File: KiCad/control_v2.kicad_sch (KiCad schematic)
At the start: 22 parts, among them J1 DE9_Pins, J2 DE9_Pins, J3 Conn_01x05, U1 FDC2214, U2 SN65HVD230, U3 PIC24HJ128GP502, Y1 Crystal

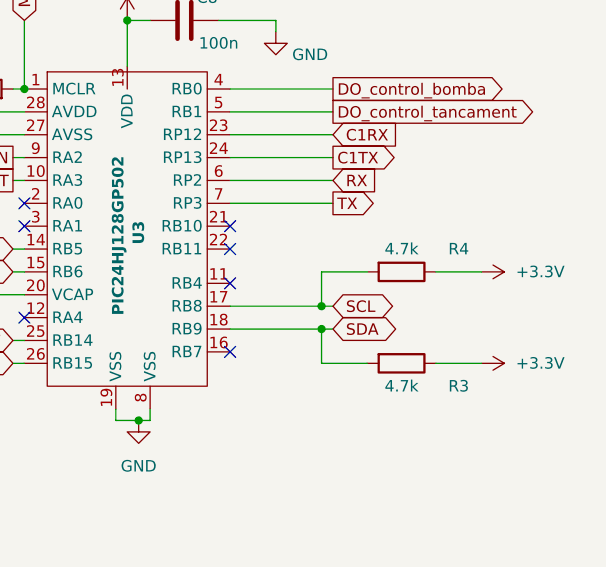
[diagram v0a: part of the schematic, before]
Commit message: commit por alfred
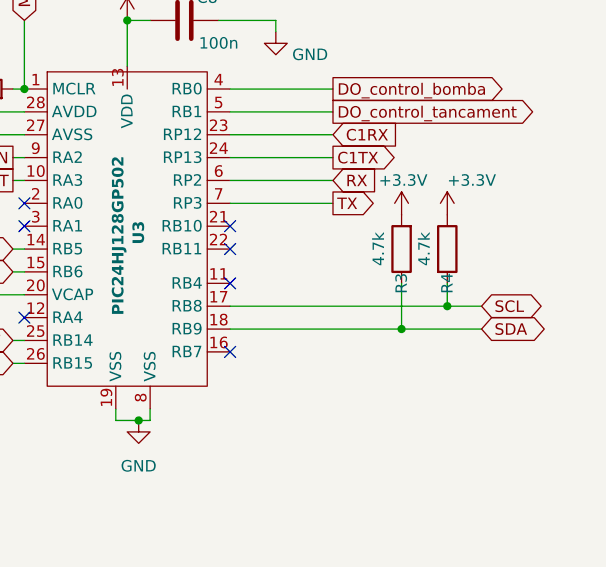
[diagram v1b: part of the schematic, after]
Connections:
- net +3.3V: now also R3.2; no longer R3.1
- net SDA: now also R3.1; no longer R3.2
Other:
- moved on the sheet: R3, R4
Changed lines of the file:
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@@
 	)
 	(junction
-		(at 231.14 68.58)
-		(diameter 0)
-		(color 0 0 0 0)
-	)
-	(junction
 		(at 100.33 60.96)
 		(diameter 0)
@@
 	)
 	(junction
+		(at 240.03 68.58)
+		(diameter 0)
+		(color 0 0 0 0)
+	)
+	(junction
 		(at 217.17 123.19)
 		(diameter 0)
@@
 	)
 	(junction
-		(at 231.14 66.04)
+		(at 245.11 66.04)
 		(diameter 0)
 		(color 0 0 0 0)
@@
 	(wire
 		(pts
-			(xy 236.22 72.39) (xy 231.14 72.39)
-		)
-		(stroke
-			(width 0)
-			(type default)
-		)
-	)
-	(wire
-		(pts
 			(xy 208.28 78.74) (xy 210.82 78.74)
 		)
@@
 	(wire
 		(pts
-			(xy 236.22 62.23) (xy 231.14 62.23)
-		)
-		(stroke
-			(width 0)
-			(type default)
-		)
-	)
-	(wire
-		(pts
-			(xy 243.84 72.39) (xy 248.92 72.39)
+			(xy 160.02 120.65) (xy 165.1 120.65)
 		)
 		(stroke
@@
 	(wire
 		(pts
-			(xy 160.02 120.65) (xy 165.1 120.65)
+			(xy 240.03 68.58) (xy 248.92 68.58)
 		)
 		(stroke
@@
 	(wire
 		(pts
-			(xy 220.98 66.04) (xy 231.14 66.04)
+			(xy 220.98 66.04) (xy 245.11 66.04)
 		)
 		(stroke
@@
 	(wire
 		(pts
+			(xy 245.11 63.5) (xy 245.11 66.04)
+		)
+		(stroke
+			(width 0)
+			(type default)
+		)
+	)
+	(wire
+		(pts
 			(xy 219.71 34.29) (xy 226.06 34.29)
 		)
@@
 	(wire
 		(pts
-			(xy 220.98 49.53) (xy 232.41 49.53)
+			(xy 245.11 66.04) (xy 248.92 66.04)
 		)
 		(stroke
@@
 	(wire
 		(pts
-			(xy 184.15 40.64) (xy 184.15 44.45)
+			(xy 220.98 49.53) (xy 232.41 49.53)
 		)
 		(stroke
@@
 	(wire
 		(pts
-			(xy 184.15 46.99) (xy 184.15 48.26)
+			(xy 184.15 40.64) (xy 184.15 44.45)
 		)
 		(stroke
@@
 	(wire
 		(pts
-			(xy 243.84 62.23) (xy 248.92 62.23)
+			(xy 184.15 46.99) (xy 184.15 48.26)
 		)
 		(stroke
@@
 	(wire
 		(pts
-			(xy 220.98 68.58) (xy 231.14 68.58)
+			(xy 220.98 68.58) (xy 240.03 68.58)
 		)
 		(stroke
@@
 	(wire
 		(pts
+			(xy 240.03 63.5) (xy 240.03 68.58)
+		)
+		(stroke
+			(width 0)
+			(type default)
+		)
+	)
+	(wire
+		(pts
 			(xy 160.02 128.27) (xy 165.1 128.27)
 		)
@@
 		)
 	)
-	(wire
-		(pts
-			(xy 231.14 66.04) (xy 232.41 66.04)
-		)
-		(stroke
-			(width 0)
-			(type default)
-		)
-	)
 	(bus
 		(pts
@@
 	(wire
 		(pts
-			(xy 231.14 68.58) (xy 231.14 72.39)
-		)
-		(stroke
-			(width 0)
-			(type default)
-		)
-	)
-	(wire
-		(pts
 			(xy 102.87 151.13) (xy 105.41 151.13)
 		)
@@
 	(wire
 		(pts
-			(xy 231.14 68.58) (xy 232.41 68.58)
-		)
-		(stroke
-			(width 0)
-			(type default)
-		)
-	)
-	(wire
-		(pts
 			(xy 100.33 60.96) (xy 106.68 60.96)
 		)
@@
 	(wire
 		(pts
-			(xy 231.14 62.23) (xy 231.14 66.04)
-		)
-		(stroke
-			(width 0)
-			(type default)
-		)
-	)
-	(wire
-		(pts
 			(xy 96.52 53.34) (xy 100.33 53.34)
 		)
@@
 	(global_label "SDA"
 		(shape bidirectional)
-		(at 232.41 68.58 0)
+		(at 248.92 68.58 0)
 		(fields_autoplaced yes)
 		(effects
@@
 		)
 		(property "Intersheetrefs" "${INTERSHEET_REFS}"
-			(at 240.0746 68.58 0)
+			(at 256.5846 68.58 0)
 			(effects
 				(font
@@
 	(global_label "SCL"
 		(shape bidirectional)
-		(at 232.41 66.04 0)
+		(at 248.92 66.04 0)
 		(fields_autoplaced yes)
 		(effects
@@
 		)
 		(property "Intersheetrefs" "${INTERSHEET_REFS}"
-			(at 240.0141 66.04 0)
+			(at 256.5241 66.04 0)
 			(effects
 				(font
@@
 	(symbol
 		(lib_id "power:+3.3V")
-		(at 248.92 62.23 270)
+		(at 245.11 55.88 0)
 		(unit 1)
 		(exclude_from_sim no)
@@
 		(on_board yes)
 		(dnp no)
-		(fields_autoplaced yes)
 		(property "Reference" "#PWR018"
-			(at 245.11 62.23 0)
+			(at 245.11 59.69 0)
 			(effects
 				(font
@@
 		)
 		(property "Value" "+3.3V"
-			(at 252.73 62.2299 90)
+			(at 245.11 52.07 0)
 			(effects
 				(font
@@
 		)
 		(property "Footprint" ""
-			(at 248.92 62.23 0)
+			(at 245.11 55.88 0)
 			(effects
 				(font
@@
 		)
 		(property "Datasheet" ""
-			(at 248.92 62.23 0)
+			(at 245.11 55.88 0)
 			(effects
 				(font
@@
 		)
 		(property "Description" "Power symbol creates a global label with name \"+3.3V\""
-			(at 248.92 62.23 0)
+			(at 245.11 55.88 0)
 			(effects
 				(font
@@
 	(symbol
 		(lib_id "power:+3.3V")
-		(at 248.92 72.39 270)
+		(at 240.03 55.88 0)
 		(unit 1)
 		(exclude_from_sim no)
@@
 		(on_board yes)
 		(dnp no)
-		(fields_autoplaced yes)
 		(property "Reference" "#PWR017"
-			(at 245.11 72.39 0)
+			(at 240.03 59.69 0)
 			(effects
 				(font
@@
 		)
 		(property "Value" "+3.3V"
-			(at 252.73 72.3899 90)
+			(at 237.49 52.07 0)
 			(effects
 				(font
@@
 		)
 		(property "Footprint" ""
-			(at 248.92 72.39 0)
+			(at 240.03 55.88 0)
 			(effects
 				(font
@@
 		)
 		(property "Datasheet" ""
-			(at 248.92 72.39 0)
+			(at 240.03 55.88 0)
 			(effects
 				(font
@@
 		)
 		(property "Description" "Power symbol creates a global label with name \"+3.3V\""
-			(at 248.92 72.39 0)
+			(at 240.03 55.88 0)
 			(effects
 				(font
@@
 	(symbol
 		(lib_id "Device:R")
-		(at 240.03 72.39 270)
+		(at 240.03 59.69 180)
 		(unit 1)
 		(exclude_from_sim no)
@@
 		(dnp no)
 		(property "Reference" "R3"
-			(at 246.38 74.93 90)
+			(at 240.03 63.5 90)
 			(effects
 				(font
@@
 		)
 		(property "Value" "4.7k"
-			(at 240.03 74.93 90)
+			(at 237.49 59.69 90)
 			(effects
 				(font
@@
 		)
 		(property "Footprint" ""
-			(at 240.03 70.612 90)
+			(at 241.808 59.69 90)
 			(effects
 				(font
@@
 		)
 		(property "Datasheet" "~"
-			(at 240.03 72.39 0)
+			(at 240.03 59.69 0)
 			(effects
 				(font
@@
 		)
 		(property "Description" "Resistor"
-			(at 240.03 72.39 0)
+			(at 240.03 59.69 0)
 			(effects
 				(font
@@
 	(symbol
 		(lib_id "Device:R")
-		(at 240.03 62.23 270)
+		(at 245.11 59.69 0)
 		(unit 1)
 		(exclude_from_sim no)
@@
 		(dnp no)
 		(property "Reference" "R4"
-			(at 246.38 59.69 90)
+			(at 245.11 63.5 90)
 			(effects
 				(font
@@
 		)
 		(property "Value" "4.7k"
-			(at 240.03 59.69 90)
+			(at 242.57 59.69 90)
 			(effects
 				(font
@@
 		)
 		(property "Footprint" ""
-			(at 240.03 60.452 90)
+			(at 243.332 59.69 90)
 			(effects
 				(font
@@
 		)
 		(property "Datasheet" "~"
-			(at 240.03 62.23 0)
+			(at 245.11 59.69 0)
 			(effects
 				(font
@@
 		)
 		(property "Description" "Resistor"
-			(at 240.03 62.23 0)
+			(at 245.11 59.69 0)
 			(effects
 				(font
